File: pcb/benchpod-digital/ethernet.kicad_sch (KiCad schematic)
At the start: 37 parts, among them J7 HR911105A_C12074, U6 LAN8742AI-CZ-TR, Y1 6pF ±10ppm SMD2016-4P Crystal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

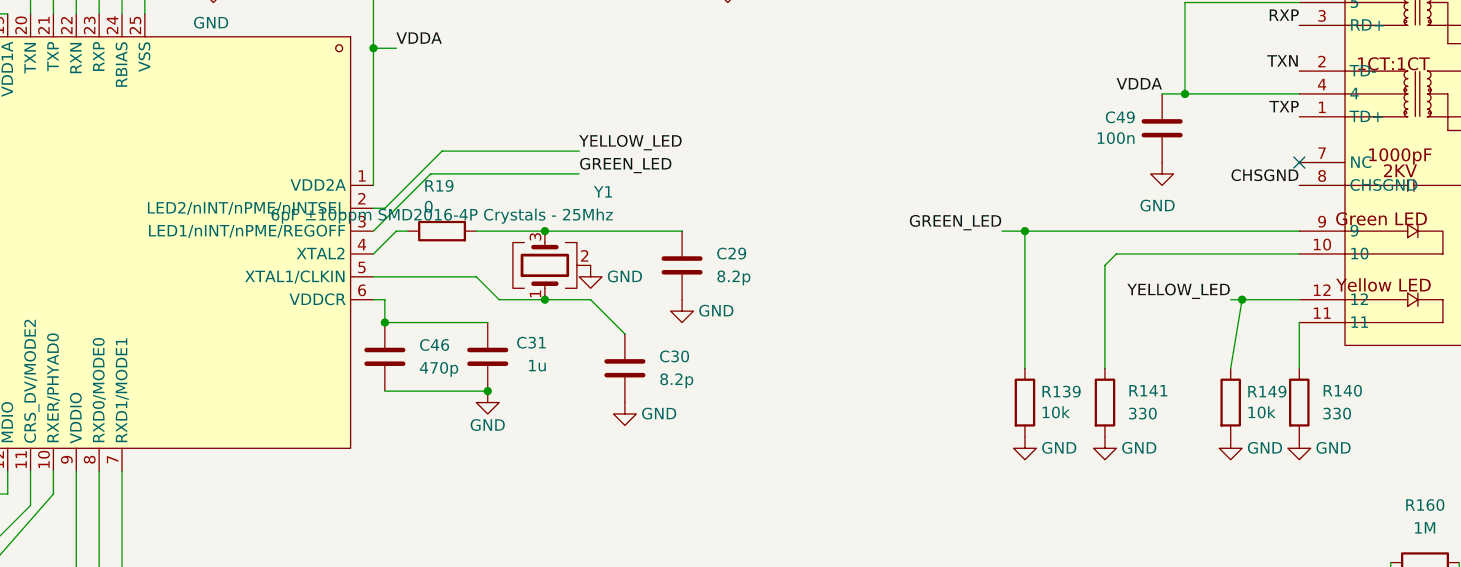
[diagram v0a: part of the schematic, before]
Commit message: signal improvements
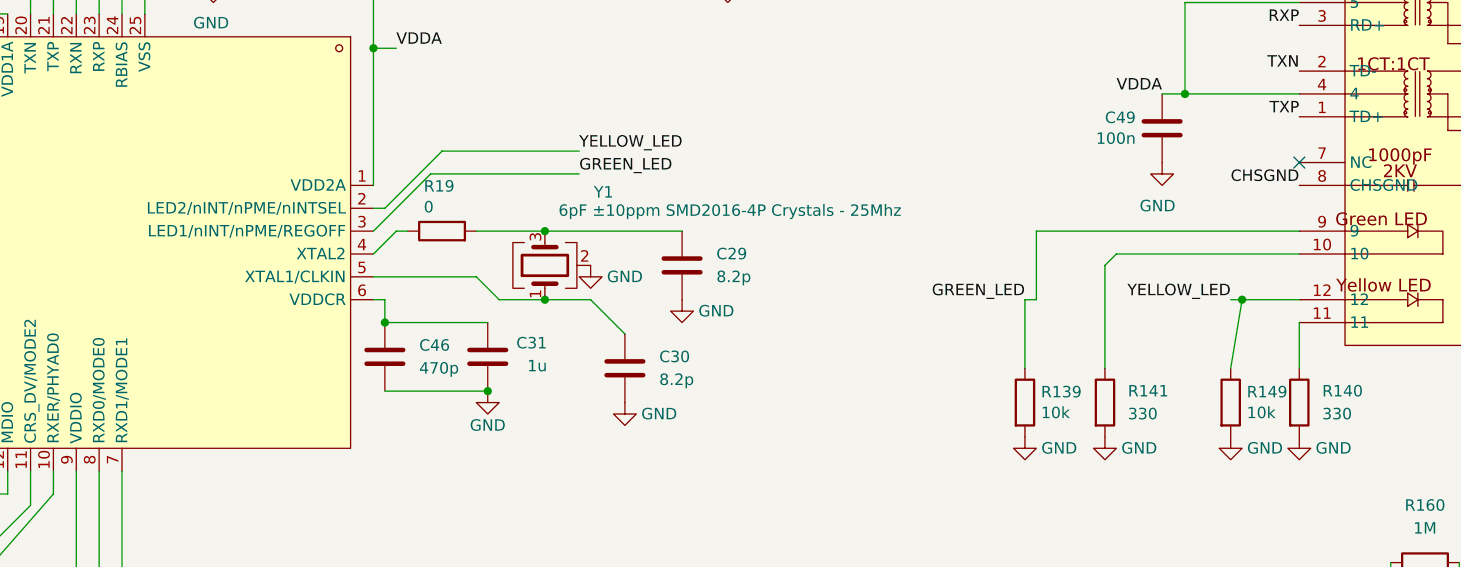
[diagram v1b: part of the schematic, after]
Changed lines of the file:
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@@
 	)
 	(junction
-		(at 184.15 72.39)
-		(diameter 0)
-		(color 0 0 0 0)
-	)
-	(junction
 		(at 81.28 20.32)
 		(diameter 0)
@@
 	(wire
 		(pts
-			(xy 184.15 72.39) (xy 214.63 72.39)
+			(xy 184.15 80.01) (xy 185.42 80.01)
 		)
 		(stroke
@@
 	(wire
 		(pts
-			(xy 181.61 72.39) (xy 184.15 72.39)
-		)
-		(stroke
-			(width 0)
-			(type default)
-		)
-	)
-	(wire
-		(pts
 			(xy 130.81 72.39) (xy 146.05 72.39)
 		)
@@
 	(wire
 		(pts
+			(xy 185.42 80.01) (xy 185.42 72.39)
+		)
+		(stroke
+			(width 0)
+			(type default)
+		)
+	)
+	(wire
+		(pts
 			(xy 214.63 87.63) (xy 214.63 82.55)
 		)
@@
 	(wire
 		(pts
-			(xy 184.15 87.63) (xy 184.15 72.39)
+			(xy 184.15 87.63) (xy 184.15 80.01)
 		)
 		(stroke
@@
 	(wire
 		(pts
+			(xy 185.42 72.39) (xy 214.63 72.39)
+		)
+		(stroke
+			(width 0)
+			(type default)
+		)
+	)
+	(wire
+		(pts
 			(xy 113.03 80.01) (xy 113.03 82.55)
 		)
@@
 	)
 	(label "GREEN_LED"
-		(at 181.61 72.39 180)
+		(at 184.15 80.01 180)
 		(effects
 			(font
@@
 		)
 		(property "Value" "6pF ±10ppm SMD2016-4P Crystals  - 25Mhz"
-			(at 138.43 70.612 90)
+			(at 170.434 70.104 90)
 			(show_name no)
 			(do_not_autoplace no)
